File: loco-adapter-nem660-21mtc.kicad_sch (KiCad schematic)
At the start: 1 part, among them J1201 Conn_02x11_Odd_Even

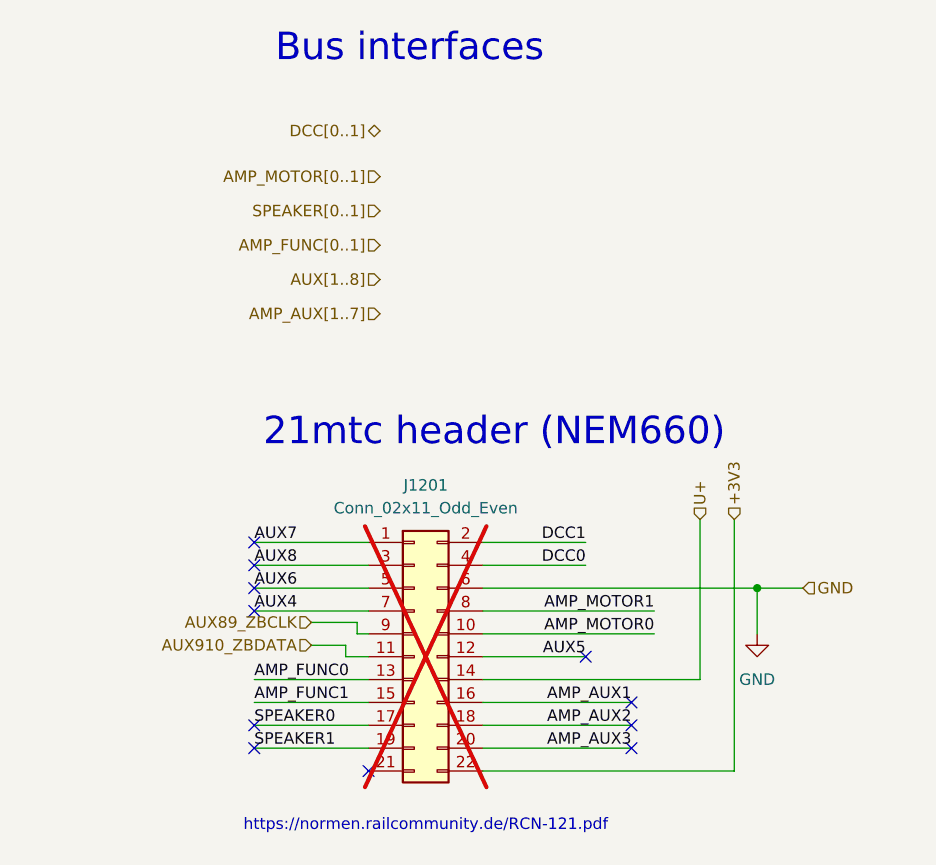
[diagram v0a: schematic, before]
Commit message: Add - plux16 integration v0.9
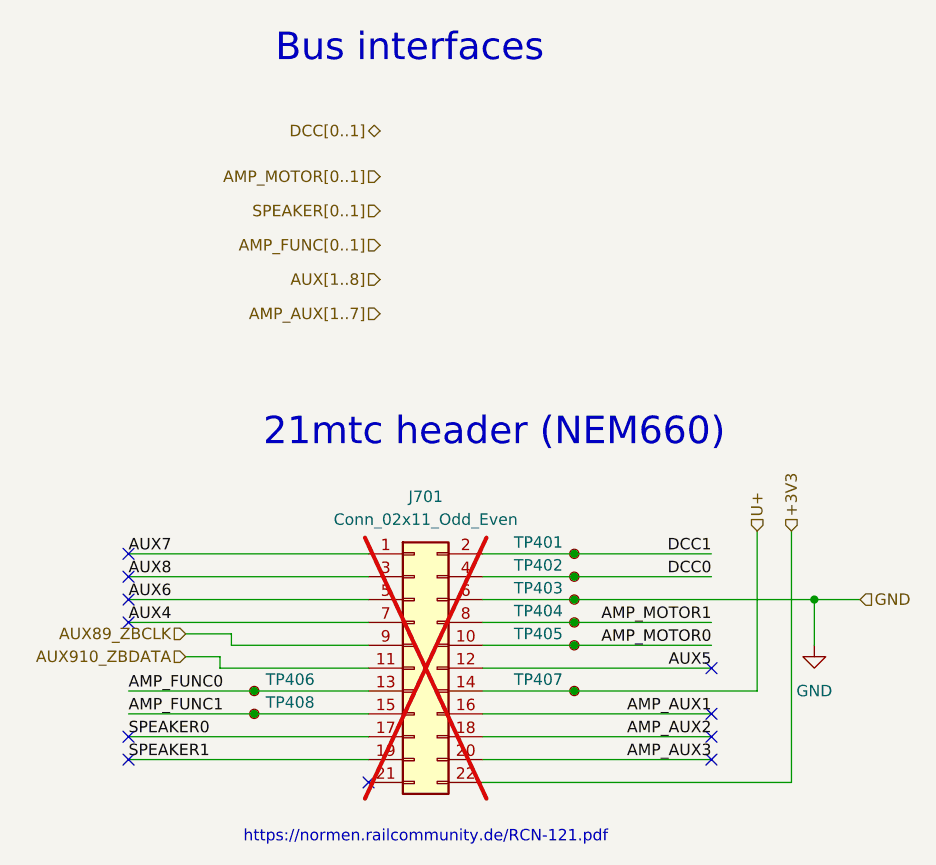
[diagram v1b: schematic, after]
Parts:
- added TP401, TP402, TP403, TP404, TP405, TP406, TP407, TP408: ~, TestPoint:TestPoint_Pad_D1.0mm, symbol Connector:TestPoint_Small
- J701: renamed from J1201; OLI_ID (none) -> MTC21_02x11_1.27
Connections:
- net AMP_FUNC0: now also TP406.1
- net AMP_FUNC1: now also TP408.1
- net AMP_MOTOR0: now also TP405.1
- net AMP_MOTOR1: now also TP404.1
- net DCC0: now also TP402.1
- net DCC1: now also TP401.1
- net GND: now also TP403.1
- net U+: now also TP407.1
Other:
- company: (none) -> Chatelain Engineering, Bern - CH
- title: (none) -> xDuinoRail - RailcomDecoder - Development Kit "Hermes"
- moved on the sheet: J701
